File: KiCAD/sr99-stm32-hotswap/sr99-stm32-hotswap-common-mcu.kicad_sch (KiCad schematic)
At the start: 65 parts, among them J1 UDB, J3 TC2030_SWD, J4 Conn_01x02, Q1 2N7002, Q2 2N7002, Q3 2N7002, U1 STM32G474CBTx, U2 MC74HC589AD, U3 MC74HC589AD, U4 MC74HC589AD, U5 M25C-MEM-SPI, U6 AP2112K, Y1 8Mhz SMD3225-4P

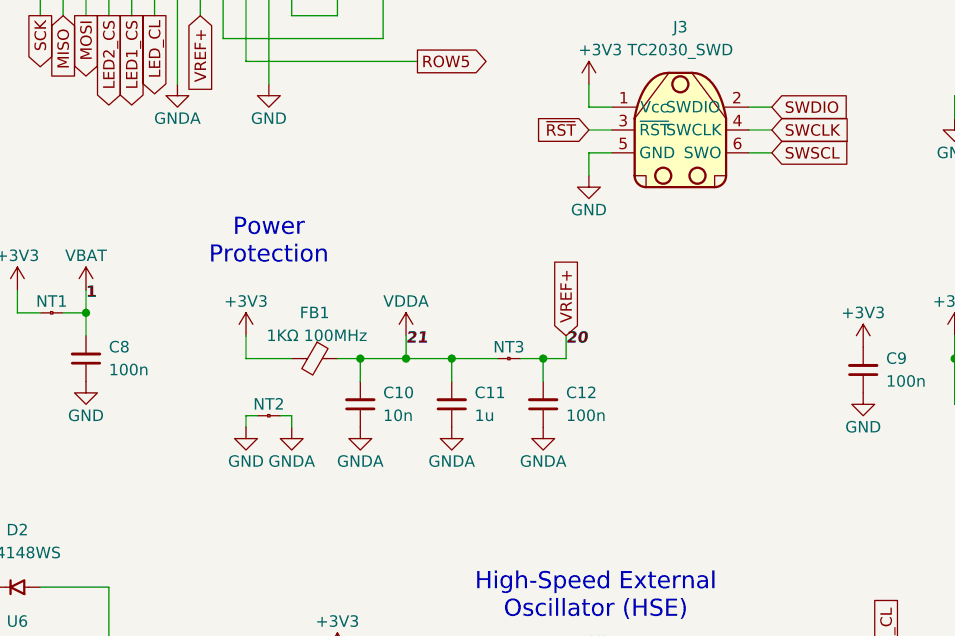
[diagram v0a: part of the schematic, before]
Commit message: .
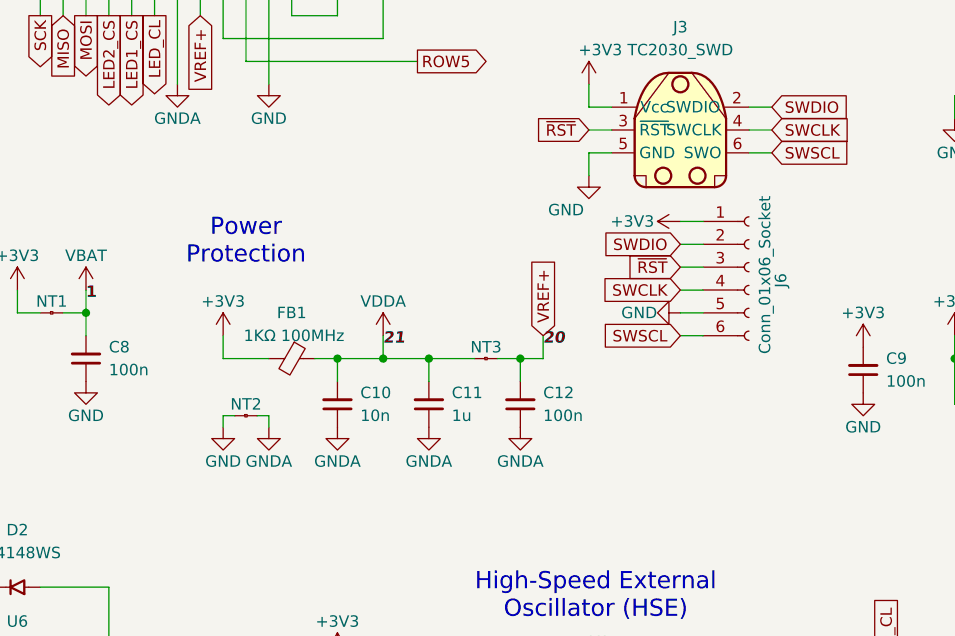
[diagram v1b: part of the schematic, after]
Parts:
- added J6: Conn_01x06_Socket, ts-kicad-lib:Tag-Connect_EC-06-IDC_P1.27mm_Vertical, symbol Connector:Conn_01x06_Socket
- J3: footprint Connector:Tag-Connect_TC2030-IDC-NL_2x03_P1.27mm_Vertical -> ts-kicad-lib:Tag-Connect_TC2030-IDC-NL_2x03_P1.27mm_Vertical
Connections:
- net +3V3: now also J6.1 (Pin_1)
- net GND: now also J6.5 (Pin_5)
- net SWCLK: now also J6.4 (Pin_4)
- net SWDIO: now also J6.2 (Pin_2)
- net SWSCL: now also J6.6 (Pin_6)
- net ~{RST}: now also J6.3 (Pin_3)
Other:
- moved on the sheet: C10, C11, C12, FB1, NT2, NT3
